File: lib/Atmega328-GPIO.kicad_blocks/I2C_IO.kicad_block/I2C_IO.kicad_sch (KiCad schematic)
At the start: 2 parts, among them J6 Conn_01x04_Socket

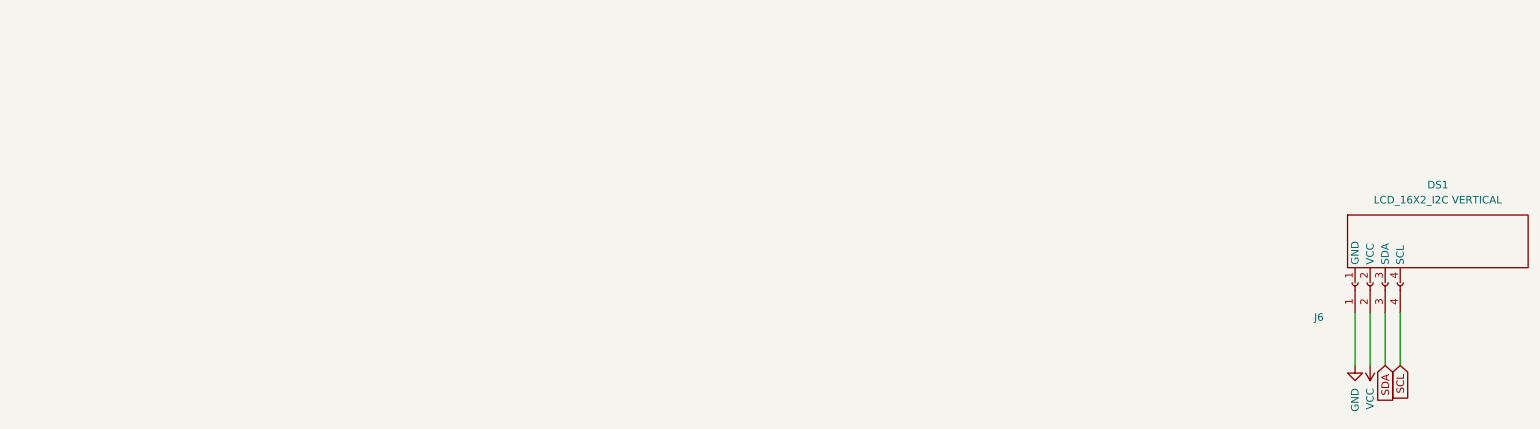
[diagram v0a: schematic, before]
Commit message: 5/21/25-1
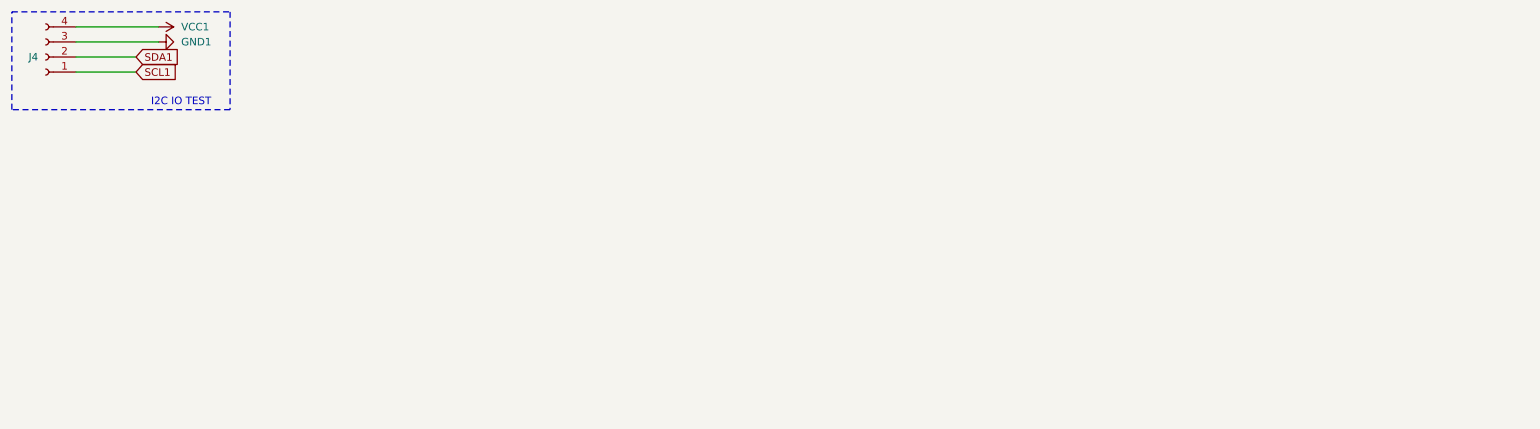
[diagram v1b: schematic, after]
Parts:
- removed DS1: LCD_16X2_I2C VERTICAL, Add_New:LCD 16X2 I2C, symbol Add_new:LCD_16X2_I2C
- removed J6: Conn_01x04_Socket, Add_New:Conn_4x1_90deg_angle, symbol Connector:Conn_01x04_Socket
- added J4: Conn_01x04_Socket, Add_New:CONN_PPTC041LFBN-RC_SUL, symbol Connector:Conn_01x04_Socket
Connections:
- new net GND1: J4.3 (Pin_3)
- new net SCL1: J4.1 (Pin_1)
- new net SDA1: J4.2 (Pin_2)
- new net VCC1: J4.4 (Pin_4)
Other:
- note added: "I2C IO TEST"
